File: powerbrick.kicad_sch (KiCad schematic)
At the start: 8 parts, among them U4 LM2596S-3.3, U7 AMS1117-3.3

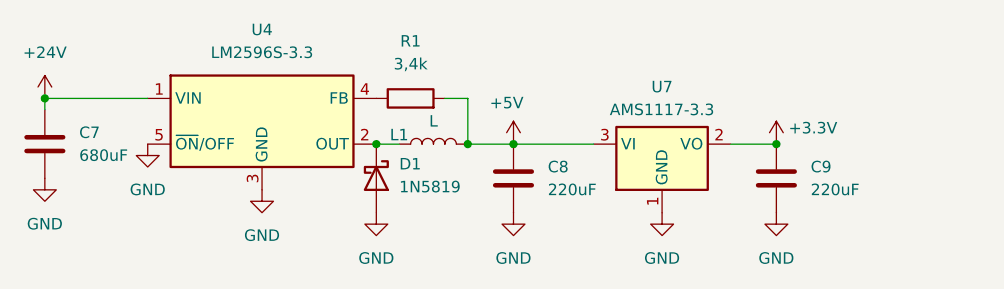
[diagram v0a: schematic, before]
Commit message: .
označení sekcí
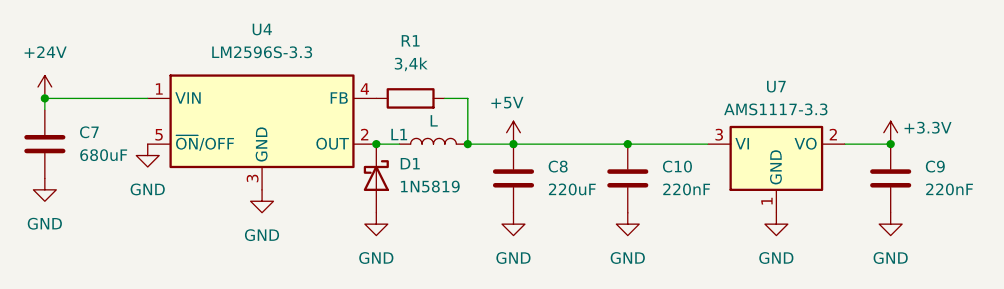
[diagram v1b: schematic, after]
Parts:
- added C10: 220nF, symbol Device:C
- C9: value 220uF -> 220nF
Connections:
- net +5V: now also C10.1
- net GND: now also C10.2
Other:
- moved on the sheet: C9, U7
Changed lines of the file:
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@@
 	)
 	(junction
-		(at 152.4 40.64)
+		(at 165.1 40.64)
+		(diameter 0)
+		(color 0 0 0 0)
+	)
+	(junction
+		(at 135.89 40.64)
 		(diameter 0)
 		(color 0 0 0 0)
@@
 	(wire
 		(pts
-			(xy 123.19 40.64) (xy 132.08 40.64)
+			(xy 123.19 40.64) (xy 135.89 40.64)
 		)
 		(stroke
@@
 	(wire
 		(pts
-			(xy 71.12 35.56) (xy 71.12 36.83)
+			(xy 135.89 40.64) (xy 144.78 40.64)
 		)
 		(stroke
@@
 	(wire
 		(pts
-			(xy 118.11 35.56) (xy 118.11 40.64)
+			(xy 71.12 35.56) (xy 71.12 36.83)
 		)
 		(stroke
@@
 	(wire
 		(pts
-			(xy 71.12 35.56) (xy 82.55 35.56)
+			(xy 118.11 35.56) (xy 118.11 40.64)
 		)
 		(stroke
@@
 	(wire
 		(pts
-			(xy 118.11 40.64) (xy 123.19 40.64)
+			(xy 71.12 35.56) (xy 82.55 35.56)
 		)
 		(stroke
@@
 	(wire
 		(pts
-			(xy 152.4 40.64) (xy 147.32 40.64)
+			(xy 118.11 40.64) (xy 123.19 40.64)
 		)
 		(stroke
@@
 		)
 	)
+	(wire
+		(pts
+			(xy 165.1 40.64) (xy 160.02 40.64)
+		)
+		(stroke
+			(width 0)
+			(type default)
+		)
+	)
 	(symbol
 		(lib_id "Device:R")
@@
 	)
 	(symbol
+		(lib_id "Device:C")
+		(at 135.89 44.45 0)
+		(unit 1)
+		(exclude_from_sim no)
+		(in_bom yes)
+		(on_board yes)
+		(dnp no)
+		(fields_autoplaced yes)
+		(property "Reference" "C10"
+			(at 139.7 43.1799 0)
+			(effects
+				(font
+					(size 1.27 1.27)
+				)
+				(justify left)
+			)
+		)
+		(property "Value" "220nF"
+			(at 139.7 45.7199 0)
+			(effects
+				(font
+					(size 1.27 1.27)
+				)
+				(justify left)
+			)
+		)
+		(property "Footprint" ""
+			(at 136.8552 48.26 0)
+			(effects
+				(font
+					(size 1.27 1.27)
+				)
+				(hide yes)
+			)
+		)
+		(property "Datasheet" "~"
+			(at 135.89 44.45 0)
+			(effects
+				(font
+					(size 1.27 1.27)
+				)
+				(hide yes)
+			)
+		)
+		(property "Description" "Unpolarized capacitor"
+			(at 135.89 44.45 0)
+			(effects
+				(font
+					(size 1.27 1.27)
+				)
+				(hide yes)
+			)
+		)
+		(pin "1"
+		)
+		(pin "2"
+		)
+		(instances
+			(project "TechStarter"
+				(path "/7ea2363f-6757-4fc6-83f2-16ce190d79d1/efa4ad20-026b-4f4f-bd8d-a347b34e01c5"
+					(reference "C10")
+					(unit 1)
+				)
+			)
+		)
+	)
+	(symbol
 		(lib_id "power:GND")
 		(at 123.19 48.26 0)
@@
 	(symbol
 		(lib_id "power:+3.3V")
-		(at 152.4 40.64 0)
+		(at 165.1 40.64 0)
 		(unit 1)
 		(exclude_from_sim no)
@@
 		(dnp no)
 		(property "Reference" "#PWR032"
-			(at 152.4 44.45 0)
+			(at 165.1 44.45 0)
 			(effects
 				(font
@@
 		)
 		(property "Value" "+3.3V"
-			(at 156.464 38.862 0)
-			(effects
-				(font
-					(size 1.27 1.27)
-				)
-			)
-		)
-		(property "Footprint" ""
-			(at 152.4 40.64 0)
+			(at 169.164 38.862 0)
+			(effects
+				(font
+					(size 1.27 1.27)
+				)
+			)
+		)
+		(property "Footprint" ""
+			(at 165.1 40.64 0)
 			(effects
 				(font
@@
 		)
 		(property "Datasheet" ""
-			(at 152.4 40.64 0)
+			(at 165.1 40.64 0)
 			(effects
 				(font
@@
 		)
 		(property "Description" "Power symbol creates a global label with name \"+3.3V\""
-			(at 152.4 40.64 0)
+			(at 165.1 40.64 0)
 			(effects
 				(font
@@
 	(symbol
 		(lib_id "power:GND")
-		(at 139.7 48.26 0)
+		(at 152.4 48.26 0)
 		(unit 1)
 		(exclude_from_sim no)
@@
 		(fields_autoplaced yes)
 		(property "Reference" "#PWR027"
-			(at 139.7 54.61 0)
+			(at 152.4 54.61 0)
 			(effects
 				(font
@@
 		)
 		(property "Value" "GND"
-			(at 139.7 53.34 0)
-			(effects
-				(font
-					(size 1.27 1.27)
-				)
-			)
-		)
-		(property "Footprint" ""
-			(at 139.7 48.26 0)
+			(at 152.4 53.34 0)
+			(effects
+				(font
+					(size 1.27 1.27)
+				)
+			)
+		)
+		(property "Footprint" ""
+			(at 152.4 48.26 0)
 			(effects
 				(font
@@
 		)
 		(property "Datasheet" ""
-			(at 139.7 48.26 0)
+			(at 152.4 48.26 0)
 			(effects
 				(font
@@
 		)
 		(property "Description" "Power symbol creates a global label with name \"GND\" , ground"
-			(at 139.7 48.26 0)
+			(at 152.4 48.26 0)
 			(effects
 				(font
@@
 	(symbol
 		(lib_id "power:GND")
-		(at 152.4 48.26 0)
+		(at 165.1 48.26 0)
 		(unit 1)
 		(exclude_from_sim no)
@@
 		(fields_autoplaced yes)
 		(property "Reference" "#PWR030"
-			(at 152.4 54.61 0)
+			(at 165.1 54.61 0)
 			(effects
 				(font
@@
 		)
 		(property "Value" "GND"
-			(at 152.4 53.34 0)
-			(effects
-				(font
-					(size 1.27 1.27)
-				)
-			)
-		)
-		(property "Footprint" ""
-			(at 152.4 48.26 0)
+			(at 165.1 53.34 0)
+			(effects
+				(font
+					(size 1.27 1.27)
+				)
+			)
+		)
+		(property "Footprint" ""
+			(at 165.1 48.26 0)
 			(effects
 				(font
@@
 		)
 		(property "Datasheet" ""
-			(at 152.4 48.26 0)
+			(at 165.1 48.26 0)
 			(effects
 				(font
@@
 		)
 		(property "Description" "Power symbol creates a global label with name \"GND\" , ground"
-			(at 152.4 48.26 0)
+			(at 165.1 48.26 0)
 			(effects
 				(font
@@
 	)
 	(symbol
+		(lib_id "power:GND")
+		(at 135.89 48.26 0)
+		(unit 1)
+		(exclude_from_sim no)
+		(in_bom yes)
+		(on_board yes)
+		(dnp no)
+		(fields_autoplaced yes)
+		(property "Reference" "#PWR057"
+			(at 135.89 54.61 0)
+			(effects
+				(font
+					(size 1.27 1.27)
+				)
+				(hide yes)
+			)
+		)
+		(property "Value" "GND"
+			(at 135.89 53.34 0)
+			(effects
+				(font
+					(size 1.27 1.27)
+				)
+			)
+		)
+		(property "Footprint" ""
+			(at 135.89 48.26 0)
+			(effects
+				(font
+					(size 1.27 1.27)
+				)
+				(hide yes)
+			)
+		)
+		(property "Datasheet" ""
+			(at 135.89 48.26 0)
+			(effects
+				(font
+					(size 1.27 1.27)
+				)
+				(hide yes)
+			)
+		)
+		(property "Description" "Power symbol creates a global label with name \"GND\" , ground"
+			(at 135.89 48.26 0)
+			(effects
+				(font
+					(size 1.27 1.27)
+				)
+				(hide yes)
+			)
+		)
+		(pin "1"
+		)
+		(instances
+			(project "TechStarter"
+				(path "/7ea2363f-6757-4fc6-83f2-16ce190d79d1/efa4ad20-026b-4f4f-bd8d-a347b34e01c5"
+					(reference "#PWR057")
+					(unit 1)
+				)
+			)
+		)
+	)
+	(symbol
 		(lib_id "Device:C")
-		(at 152.4 44.45 0)
+		(at 165.1 44.45 0)
 		(unit 1)
 		(exclude_from_sim no)
@@
 		(fields_autoplaced yes)
 		(property "Reference" "C9"
-			(at 156.21 43.1799 0)
+			(at 168.91 43.1799 0)
 			(effects
 				(font
@@
 			)
 		)
-		(property "Value" "220uF"
-			(at 156.21 45.7199 0)
+		(property "Value" "220nF"
+			(at 168.91 45.7199 0)
 			(effects
 				(font
@@
 		)
 		(property "Footprint" ""
-			(at 153.3652 48.26 0)
+			(at 166.0652 48.26 0)
 			(effects
 				(font
@@
 		)
 		(property "Datasheet" "~"
-			(at 152.4 44.45 0)
+			(at 165.1 44.45 0)
 			(effects
 				(font
@@
 		)
 		(property "Description" "Unpolarized capacitor"
-			(at 152.4 44.45 0)
+			(at 165.1 44.45 0)
 			(effects
 				(font
@@
 	(symbol
 		(lib_id "Regulator_Linear:AMS1117-3.3")
-		(at 139.7 40.64 0)
+		(at 152.4 40.64 0)
 		(unit 1)
 		(exclude_from_sim no)
@@
 		(fields_autoplaced yes)
 		(property "Reference" "U7"
-			(at 139.7 34.29 0)
+			(at 152.4 34.29 0)
 			(effects
 				(font
@@
 		)
 		(property "Value" "AMS1117-3.3"
-			(at 139.7 36.83 0)
+			(at 152.4 36.83 0)
 			(effects
 				(font
@@
 		)
 		(property "Footprint" "Package_TO_SOT_SMD:SOT-223-3_TabPin2"
-			(at 139.7 35.56 0)
+			(at 152.4 35.56 0)
 			(effects
 				(font
@@
 		)
 		(property "Datasheet" "http://www.advanced-monolithic.com/pdf/ds1117.pdf"
-			(at 142.24 46.99 0)
+			(at 154.94 46.99 0)
 			(effects
 				(font
@@
 		)
 		(property "Description" "1A Low Dropout regulator, positive, 3.3V fixed output, SOT-223"
-			(at 139.7 40.64 0)
-			(effects
-				(font
+			(at 152.4 40.64 0)
+			(effects
+				(font
